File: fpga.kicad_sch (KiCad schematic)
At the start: 65 parts, among them IC1 LFE5U-25F-6BG256C, J1 JTAG, U1 W25Q128JVP

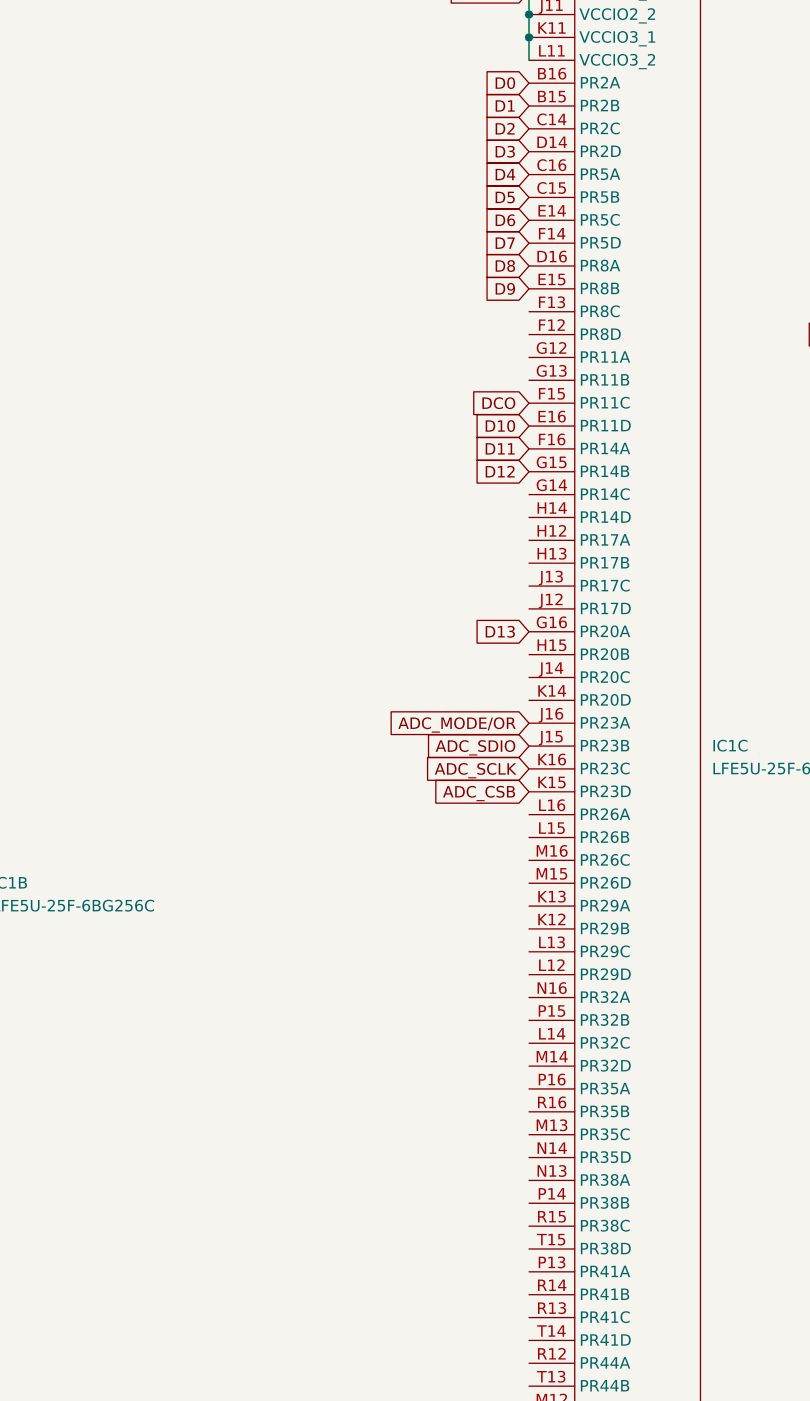
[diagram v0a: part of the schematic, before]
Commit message: dac work
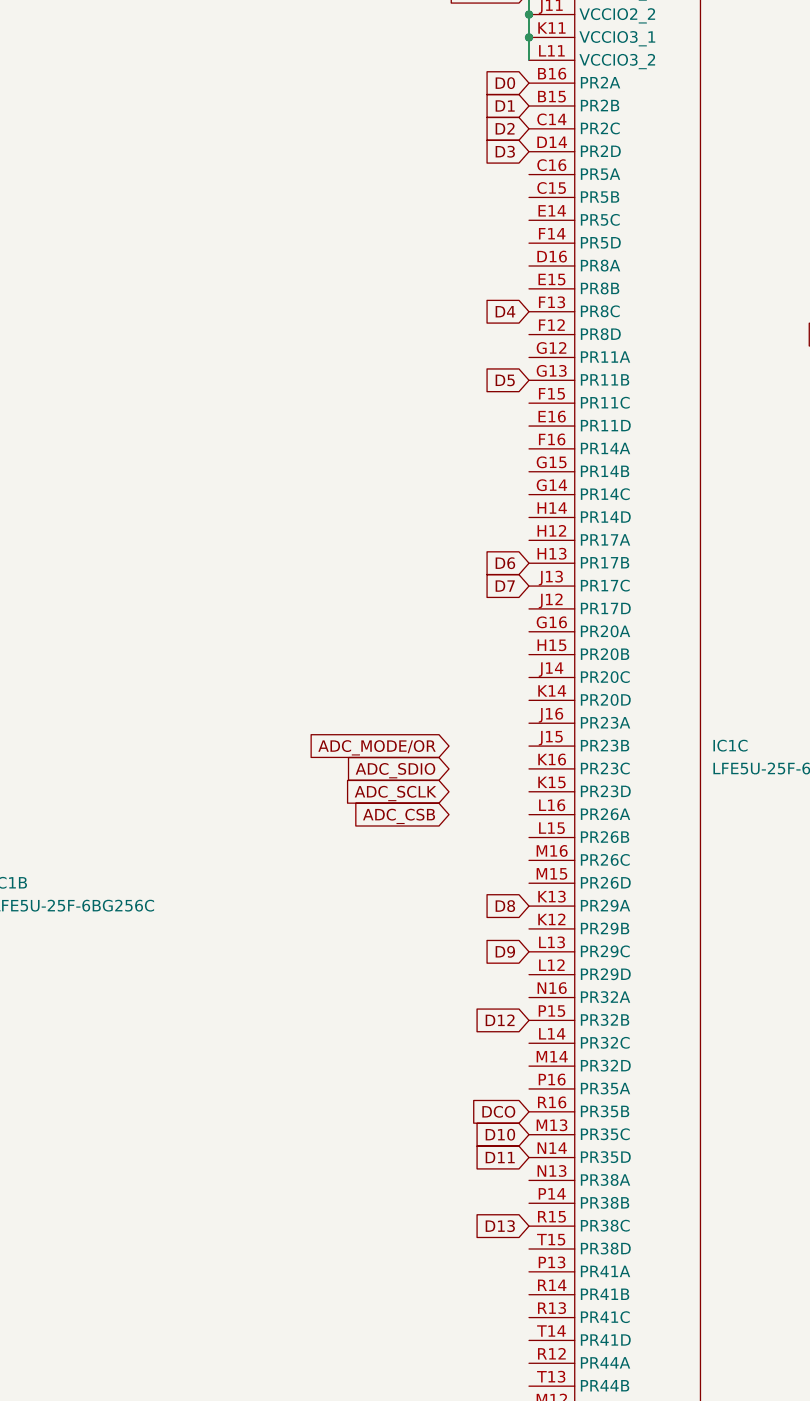
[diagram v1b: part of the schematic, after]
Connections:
- net ADC_CSB: no longer IC1.K15 (PR23D)
- net ADC_MODE/OR: no longer IC1.J16 (PR23A)
- net ADC_SCLK: no longer IC1.K16 (PR23C)
- net ADC_SDIO: no longer IC1.J15 (PR23B)
- net D10: now also IC1.M13 (PR35C); no longer IC1.E16 (PR11D)
- net D11: now also IC1.N14 (PR35D); no longer IC1.F16 (PR14A)
- net D12: now also IC1.P15 (PR32B); no longer IC1.G15 (PR14B)
- net D13: now also IC1.R15 (PR38C); no longer IC1.G16 (PR20A)
- net D4: now also IC1.F13 (PR8C); no longer IC1.C16 (PR5A)
- net D5: now also IC1.G13 (PR11B); no longer IC1.C15 (PR5B)
- net D6: now also IC1.H13 (PR17B); no longer IC1.E14 (PR5C)
- net D7: now also IC1.J13 (PR17C); no longer IC1.F14 (PR5D)
- net D8: now also IC1.K13 (PR29A); no longer IC1.D16 (PR8A)
- net D9: now also IC1.L13 (PR29C); no longer IC1.E15 (PR8B)
- net DCO: now also IC1.R16 (PR35B); no longer IC1.F15 (PR11C)
